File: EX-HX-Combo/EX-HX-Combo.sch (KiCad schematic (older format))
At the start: 46 parts, among them CN1 DB9 Male, J1 IDE_CONNECTOR, J2 Bus_Tandy_Plus, J3 Bus_Tandy_Plus_Through, SW1 SW_DIP_x10, U1 BIOS FLASH, U2 74HCT245, U3 1.8432 MHz, U4 DS1315, U5 AS6C4008-55PCN, U6 16C550, U7 GD75232N, U8 GAL16V8, U9 GAL16V8, Y1 32.768 kHz

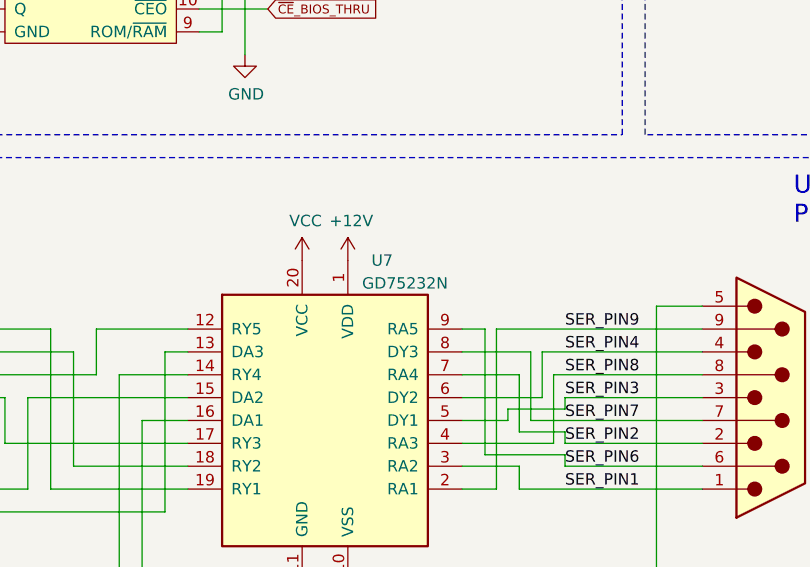
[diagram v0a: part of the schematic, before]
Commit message: EX-HX-Combo: More work preparing for JLCPCB assembly.
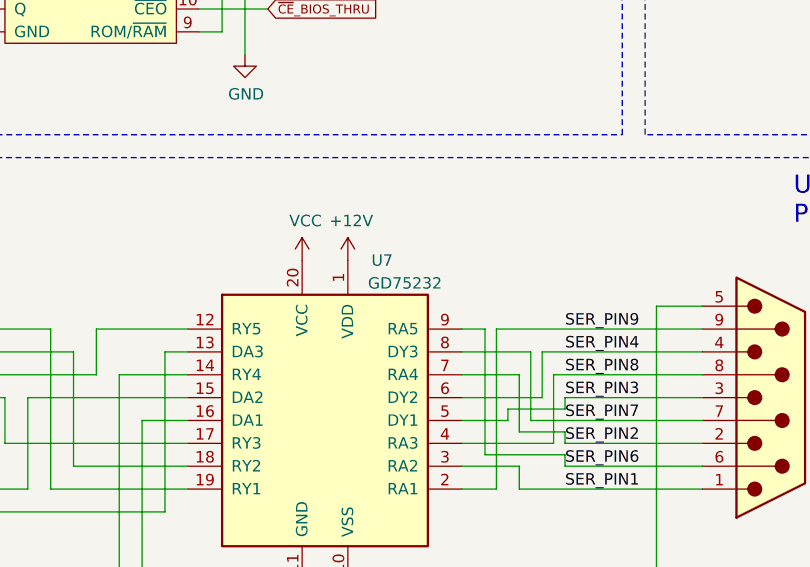
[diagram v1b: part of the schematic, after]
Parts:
- BAT1: LCSC (none) -> C964758; Part options (none) -> C964756, C964758, C964764, C964762, C70377, C964760
- C1, C10, C11, C2, C3, C4, C5, C6, C7, C8, C9: LCSC (none) -> C24497
- R1, R2, R3, R4, R5, R6, R7: LCSC (none) -> C17902
- U1, U5: LCSC (none) -> C146583; Part options (none) -> C72122, C146583, C2331
- U2, U8, U9: LCSC (none) -> C72118; Part options (none) -> C72118, C132507, C2328
- U3: LCSC (none) -> C386895
- U4: LCSC (none) -> C72115; Part options (none) -> C72115, C146580, C2326
- U6: LCSC (none) -> C181382; Part options (none) -> C181382, C2692304, C84320, C352984
- U7: value GD75232N -> GD75232; LCSC (none) -> C6662
- Y1: LCSC (none) -> C182062; Part options (none) -> C182062, C127496
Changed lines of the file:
@@
 F 3 "http://ww1.microchip.com/downloads/en/DeviceDoc/25022B.pdf" H 13850 2700 50  0001 C CNN
 F 4 "SST39SF010, SST39SF020, SST39SF040 or similar" H 13850 3789 50  0000 C CNN "Note"
+F 5 "C146583" H 13850 2400 50  0001 C CNN "LCSC"
+F 6 "C72122, C146583, C2331" H 13850 2400 50  0001 C CNN "Part options"
 	1    13850 2400
 	1    0    0    -1
@@
 F 2 "Capacitor_SMD:C_1206_3216Metric" H 8388 7550 50  0001 C CNN
 F 3 "~" H 8350 7700 50  0001 C CNN
+F 4 " C24497" H 8350 7700 50  0001 C CNN "LCSC"
 	1    8350 7700
 	1    0    0    -1
@@
 F 2 "Capacitor_SMD:C_1206_3216Metric" H 8888 7550 50  0001 C CNN
 F 3 "~" H 8850 7700 50  0001 C CNN
+F 4 " C24497" H 8850 7700 50  0001 C CNN "LCSC"
 	1    8850 7700
 	1    0    0    -1
@@
 F 2 "Package_DIP:DIP-20_W7.62mm_Socket" H 10600 2200 50  0001 C CNN
 F 3 "http://www.ti.com/lit/gpn/sn74LS245" H 10600 2200 50  0001 C CNN
+F 4 "C72118" H 10600 2200 50  0001 C CNN "LCSC"
+F 5 "C72118, C132507, C2328" H 10600 2200 50  0001 C CNN "Part options"
 	1    10600 2200
 	1    0    0    -1
@@
 F 2 "Battery:BatteryHolder_Keystone_1060_1x2032" V 2300 6310 50  0001 C CNN
 F 3 "~" V 2300 6310 50  0001 C CNN
+F 4 "C964758" H 2300 6250 50  0001 C CNN "LCSC"
+F 5 "C964756, C964758, C964764, C964762, C70377, C964760" H 2300 6250 50  0001 C CNN "Part options"
 	1    2300 6250
 	1    0    0    -1
@@
 F 2 "Crystal:Crystal_C38-LF_D3.0mm_L8.0mm_Horizontal" H 2300 5500 50  0001 C CNN
 F 3 "~" H 2300 5500 50  0001 C CNN
+F 4 "C182062" V 2300 5500 50  0001 C CNN "LCSC"
+F 5 "C182062, C127496" V 2300 5500 50  0001 C CNN "Part options"
 	1    2300 5500
 	0    1    1    0
@@
 F 2 "Package_DIP:DIP-16_W7.62mm_Socket" H 3800 5450 50  0001 C CNN
 F 3 "" H 3800 5450 50  0001 C CNN
+F 4 "C72115" H 3800 5450 50  0001 C CNN "LCSC"
+F 5 "C72115, C146580, C2326" H 3800 5450 50  0001 C CNN "Part options"
 	1    3800 5450
 	1    0    0    -1
@@
 F 2 "Package_DIP:DIP-32_W15.24mm_Socket" H 13650 5700 50  0001 C CNN
 F 3 "https://www.alliancememory.com/wp-content/uploads/pdf/AS6C4008.pdf" H 13650 5700 50  0001 C CNN
+F 4 "C146583" H 13650 5600 50  0001 C CNN "LCSC"
+F 5 "C72122, C146583, C2331" H 13650 5600 50  0001 C CNN "Part options"
 	1    13650 5600
 	1    0    0    -1
@@
 F 2 "Capacitor_SMD:C_1206_3216Metric" H 10388 7550 50  0001 C CNN
 F 3 "~" H 10350 7700 50  0001 C CNN
+F 4 " C24497" H 10350 7700 50  0001 C CNN "LCSC"
 	1    10350 7700
 	1    0    0    -1
@@
 F 2 "Capacitor_SMD:C_1206_3216Metric" H 9888 7550 50  0001 C CNN
 F 3 "~" H 9850 7700 50  0001 C CNN
+F 4 " C24497" H 9850 7700 50  0001 C CNN "LCSC"
 	1    9850 7700
 	1    0    0    -1
@@
 F 2 "Capacitor_SMD:C_1206_3216Metric" H 9388 7550 50  0001 C CNN
 F 3 "~" H 9350 7700 50  0001 C CNN
+F 4 " C24497" H 9350 7700 50  0001 C CNN "LCSC"
 	1    9350 7700
 	1    0    0    -1
@@
 P 4850 8050
 F 0 "U7" H 5100 8750 50  0000 C CNN
-F 1 "GD75232N" H 5200 8650 50  0000 C CNN
+F 1 "GD75232" H 5200 8650 50  0000 C CNN
 F 2 "Package_SO:SOIC-20W_7.5x12.8mm_P1.27mm" H 4850 7250 50  0001 C CIN
 F 3 "http://www.ti.com/lit/ds/symlink/gd75232.pdf" H 4350 8050 50  0001 C CNN
+F 4 "C6662" H 4850 8050 50  0001 C CNN "LCSC"
 	1    4850 8050
 	1    0    0    -1
@@
 F 2 "Capacitor_SMD:C_1206_3216Metric" H 11438 7550 50  0001 C CNN
 F 3 "~" H 11400 7700 50  0001 C CNN
+F 4 " C24497" H 11400 7700 50  0001 C CNN "LCSC"
 	1    11400 7700
 	1    0    0    -1
@@
 F 2 "Capacitor_SMD:C_1206_3216Metric" H 11938 7550 50  0001 C CNN
 F 3 "~" H 11900 7700 50  0001 C CNN
+F 4 " C24497" H 11900 7700 50  0001 C CNN "LCSC"
 	1    11900 7700
 	1    0    0    -1
@@
 F 2 "Capacitor_SMD:C_1206_3216Metric" H 12438 7550 50  0001 C CNN
 F 3 "~" H 12400 7700 50  0001 C CNN
+F 4 " C24497" H 12400 7700 50  0001 C CNN "LCSC"
 	1    12400 7700
 	1    0    0    -1
@@
 F 2 "Capacitor_SMD:C_1206_3216Metric" H 10888 7550 50  0001 C CNN
 F 3 "~" H 10850 7700 50  0001 C CNN
+F 4 " C24497" H 10850 7700 50  0001 C CNN "LCSC"
 	1    10850 7700
 	1    0    0    -1
@@
 F 2 "Package_DIP:DIP-20_W7.62mm_Socket" H 7700 1750 50  0001 C CNN
 F 3 "" H 7700 1750 50  0001 C CNN
+F 4 "C72118" H 7700 1750 50  0001 C CNN "LCSC"
+F 5 "C72118, C132507, C2328" H 7700 1750 50  0001 C CNN "Part options"
 	1    7700 1750
 	1    0    0    -1
@@
 F 2 "Package_DIP:DIP-20_W7.62mm_Socket" H 7700 3800 50  0001 C CNN
 F 3 "" H 7700 3800 50  0001 C CNN
+F 4 "C72118" H 7700 3800 50  0001 C CNN "LCSC"
+F 5 "C72118, C132507, C2328" H 7700 3800 50  0001 C CNN "Part options"
 	1    7700 3800
 	1    0    0    -1
@@
 F 2 "Resistor_SMD:R_1206_3216Metric" V 9030 9050 50  0001 C CNN
 F 3 "~" H 9100 9050 50  0001 C CNN
+F 4 "C17902" V 9100 9050 50  0001 C CNN "LCSC"
 	1    9100 9050
 	1    0    0    -1
@@
 F 2 "Resistor_SMD:R_1206_3216Metric" V 9430 9050 50  0001 C CNN
 F 3 "~" H 9500 9050 50  0001 C CNN
+F 4 "C17902" V 9500 9050 50  0001 C CNN "LCSC"
 	1    9500 9050
 	1    0    0    -1
@@
 F 2 "Resistor_SMD:R_1206_3216Metric" V 9230 9050 50  0001 C CNN
 F 3 "~" H 9300 9050 50  0001 C CNN
+F 4 "C17902" V 9300 9050 50  0001 C CNN "LCSC"
 	1    9300 9050
 	1    0    0    -1
@@
 F 2 "Resistor_SMD:R_1206_3216Metric" V 9630 9050 50  0001 C CNN
 F 3 "~" H 9700 9050 50  0001 C CNN
+F 4 "C17902" V 9700 9050 50  0001 C CNN "LCSC"
 	1    9700 9050
 	1    0    0    -1
@@
 F 2 "Resistor_SMD:R_1206_3216Metric" V 10030 9050 50  0001 C CNN
 F 3 "~" H 10100 9050 50  0001 C CNN
+F 4 "C17902" V 10100 9050 50  0001 C CNN "LCSC"
 	1    10100 9050
 	1    0    0    -1
@@
 Wire Wire Line
 	7250 5950 7150 5950
-$Comp
-L Oscillator:SG-7050CAN U3
-U 1 1 6125B3CC
-P 7550 5950
-F 0 "U3" H 7650 6300 50  0000 L CNN
-F 1 "1.8432 MHz" H 7650 6200 50  0000 L CNN
-F 2 "Oscillator:Oscillator_SMD_SeikoEpson_SG8002CA-4Pin_7.0x5.0mm" H 8250 5600 50  0001 C CNN
-F 3 "https://support.epson.biz/td/api/doc_check.php?dl=brief_SG7050CAN&lang=en" H 7450 5950 50  0001 C CNN
-	1    7550 5950
-	1    0    0    -1
-$EndComp
 Wire Wire Line
 	7150 5650 7150 5950
@@
 F 2 "Package_QFP:LQFP-48_7x7mm_P0.5mm" H 2350 8850 50  0001 C CIN
 F 3 "http://www.ti.com/lit/ds/symlink/pc16550d.pdf" H 2350 8850 50  0001 C CNN
+F 4 "C181382" H 2350 8850 50  0001 C CNN "LCSC"
+F 5 "C181382, C2692304, C84320, C352984" H 2350 8850 50  0001 C CNN "Part options"
 	1    2350 8850
 	1    0    0    -1
@@
 F 2 "Capacitor_SMD:C_1206_3216Metric" H 12938 7550 50  0001 C CNN
 F 3 "~" H 12900 7700 50  0001 C CNN
+F 4 " C24497" H 12900 7700 50  0001 C CNN "LCSC"
 	1    12900 7700
 	1    0    0    -1
@@
 F 2 "Capacitor_SMD:C_1206_3216Metric" H 13438 7550 50  0001 C CNN
 F 3 "~" H 13400 7700 50  0001 C CNN
+F 4 " C24497" H 13400 7700 50  0001 C CNN "LCSC"
 	1    13400 7700
 	1    0    0    -1
@@
 F 2 "Resistor_SMD:R_1206_3216Metric" V 10230 9050 50  0001 C CNN
 F 3 "~" H 10300 9050 50  0001 C CNN
+F 4 "C17902" V 10300 9050 50  0001 C CNN "LCSC"
 	1    10300 9050
 	1    0    0    -1
@@
 F 2 "Resistor_SMD:R_1206_3216Metric" V 9830 9050 50  0001 C CNN
 F 3 "~" H 9900 9050 50  0001 C CNN
+F 4 "C17902" V 9900 9050 50  0001 C CNN "LCSC"
 	1    9900 9050
 	1    0    0    -1
@@
 Text GLabel 8200 1550 2    50   Input ~ 0
 A17_MAPPED
+$Comp
+L Oscillator:SG-7050CAN U3
+U 1 1 6125B3CC
+P 7550 5950
+F 0 "U3" H 7650 6300 50  0000 L CNN
+F 1 "1.8432 MHz" H 7650 6200 50  0000 L CNN
+F 2 "Oscillator:Oscillator_SMD_SeikoEpson_SG8002CA-4Pin_7.0x5.0mm" H 8250 5600 50  0001 C CNN
+F 3 "https://support.epson.biz/td/api/doc_check.php?dl=brief_SG7050CAN&lang=en" H 7450 5950 50  0001 C CNN
+F 4 "C386895" H 7550 5950 50  0001 C CNN "LCSC"
+	1    7550 5950
+	1    0    0    -1
+$EndComp
 $EndSCHEMATC
